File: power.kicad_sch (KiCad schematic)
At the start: 22 parts, among them J3 Conn_01x02, J4 USB_C_Receptacle_PowerOnly_6P, Q1 AO3401A, U1 TP4056-42-ESOP8, U11 TPS62170DSG

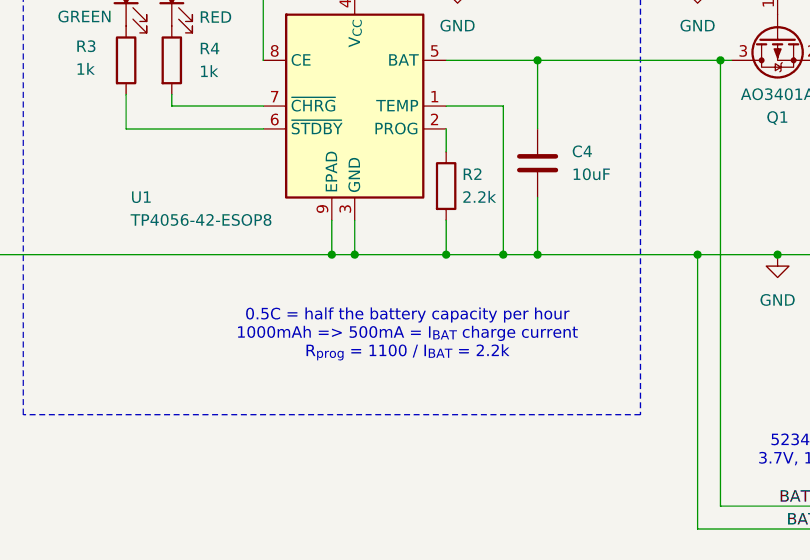
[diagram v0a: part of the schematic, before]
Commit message: remove backups, removed old chip
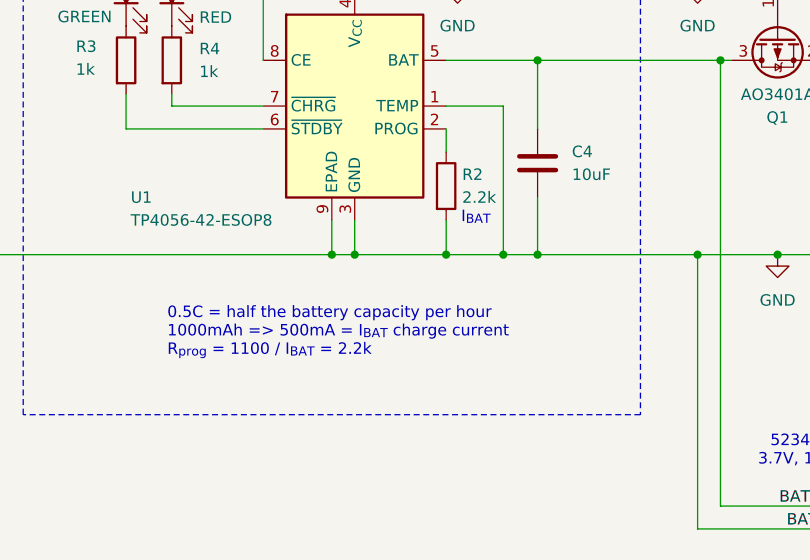
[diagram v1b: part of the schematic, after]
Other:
- note added: "I_{BAT}"
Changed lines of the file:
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@@
 		)
 	)
-	(text "0.5C = half the battery capacity per hour\n1000mAh => 500mA = I_{BAT} charge current\nR_{prog} = 1100 / I_{BAT} = 2.2k"
+	(text "I_{BAT}"
 		(exclude_from_sim no)
-		(at 123.952 113.03 0)
+		(at 131.572 100.076 0)
 		(effects
 			(font
@@
 		)
 	)
+	(text "0.5C = half the battery capacity per hour\n1000mAh => 500mA = I_{BAT} charge current\nR_{prog} = 1100 / I_{BAT} = 2.2k"
+		(exclude_from_sim no)
+		(at 97.282 112.776 0)
+		(effects
+			(font
+				(size 1.27 1.27)
+			)
+			(justify left)
+		)
+	)
